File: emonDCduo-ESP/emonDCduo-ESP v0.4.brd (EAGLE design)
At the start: 99.1 x 76.5 mm, 85 parts, among them Q1 16Mhz XT49M-2016M, U1_TQFP ATMEGA328P

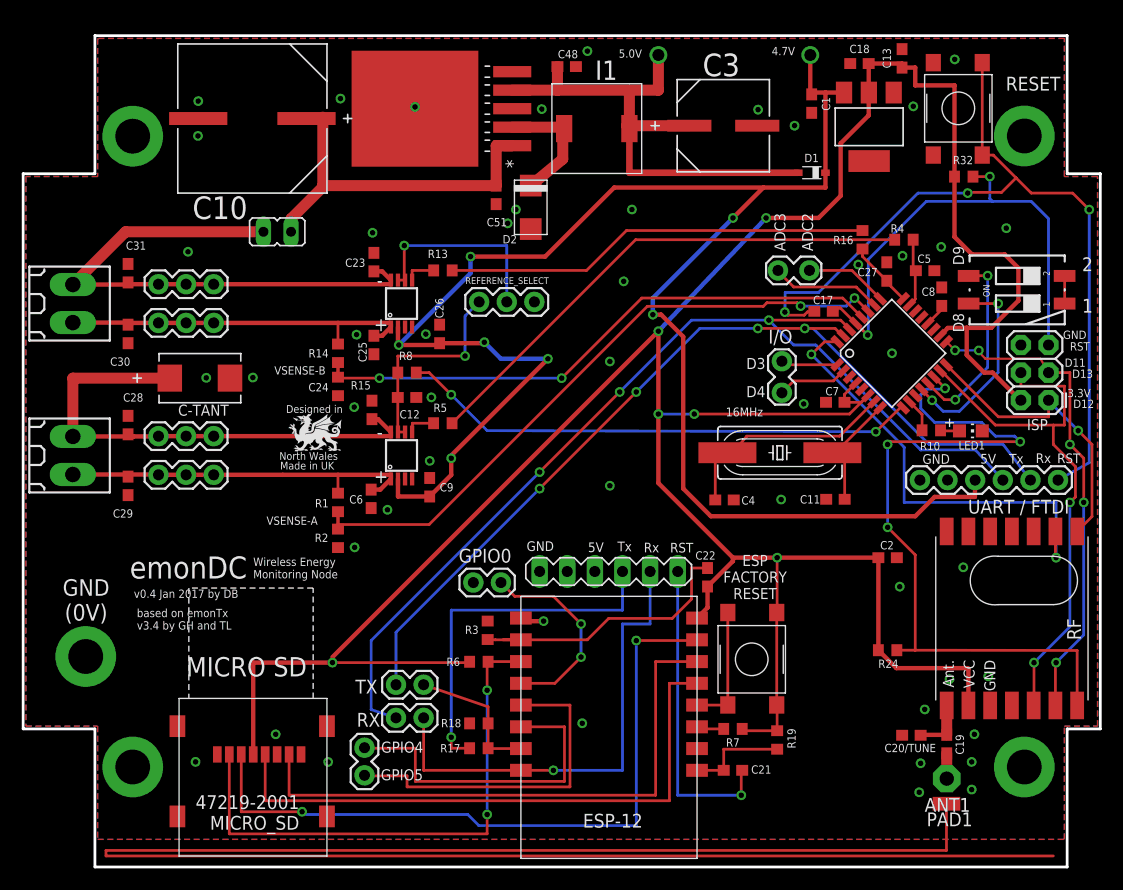
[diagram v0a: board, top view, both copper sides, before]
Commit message: updating v1.0
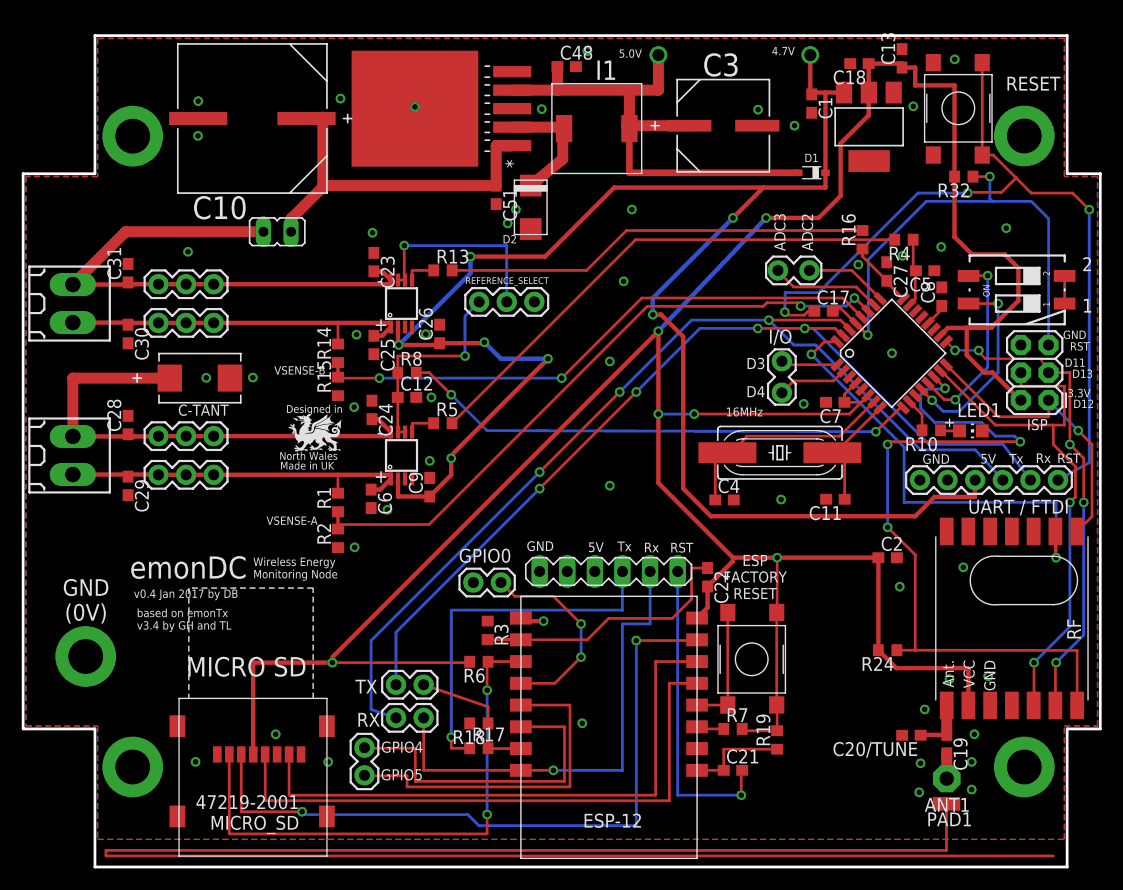
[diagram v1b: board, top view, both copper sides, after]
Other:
- board text added: "330uH"
- board text removed: "D8"
- board text removed: "D9"
